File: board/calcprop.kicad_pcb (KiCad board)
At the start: 2 copper layers, 86.6 x 171.6 mm, 126 parts, among them CON1 SD_Card, P1 BATT, P10 PROG, P2 POWER, P3 EXTBATT, P5 BACKLIGHT, P6 DISPLAY, P7 FPU, P8 EXTSPI, P9 EXTIO, SW1 KEY, SW10 KEY, SW11 KEY, SW12 KEY, SW13 KEY, SW14 KEY, SW15 KEY, SW16 KEY, SW17 KEY, SW18 KEY, SW19 KEY, SW2 KEY, SW20 KEY, SW21 KEY, SW22 KEY, SW23 KEY, SW24 KEY, SW25 KEY, SW26 KEY, SW27 KEY, SW28 KEY, SW29 KEY, SW3 KEY, SW30 KEY, SW31 KEY, SW32 KEY, SW33 KEY, SW34 KEY, SW35 KEY, SW36 KEY, SW37 KEY, SW38 KEY, SW39 KEY, SW4 KEY, SW40 KEY, SW41 KEY, SW42 KEY, SW43 KEY, SW44 KEY, SW45 KEY, SW46 KEY, SW47 KEY, SW48 KEY, SW5 KEY, SW6 KEY, SW7 KEY, SW8 KEY, SW9 KEY, U1 74LS595, U2 PROPELLER-QFN, U3 MCP3002, U4 LTC3525-3.3, U5 24LC512, U6 SST25VF080, U7 MCP23S17, U8 23xx1024, U9 23xx1024, Y1 5MHz

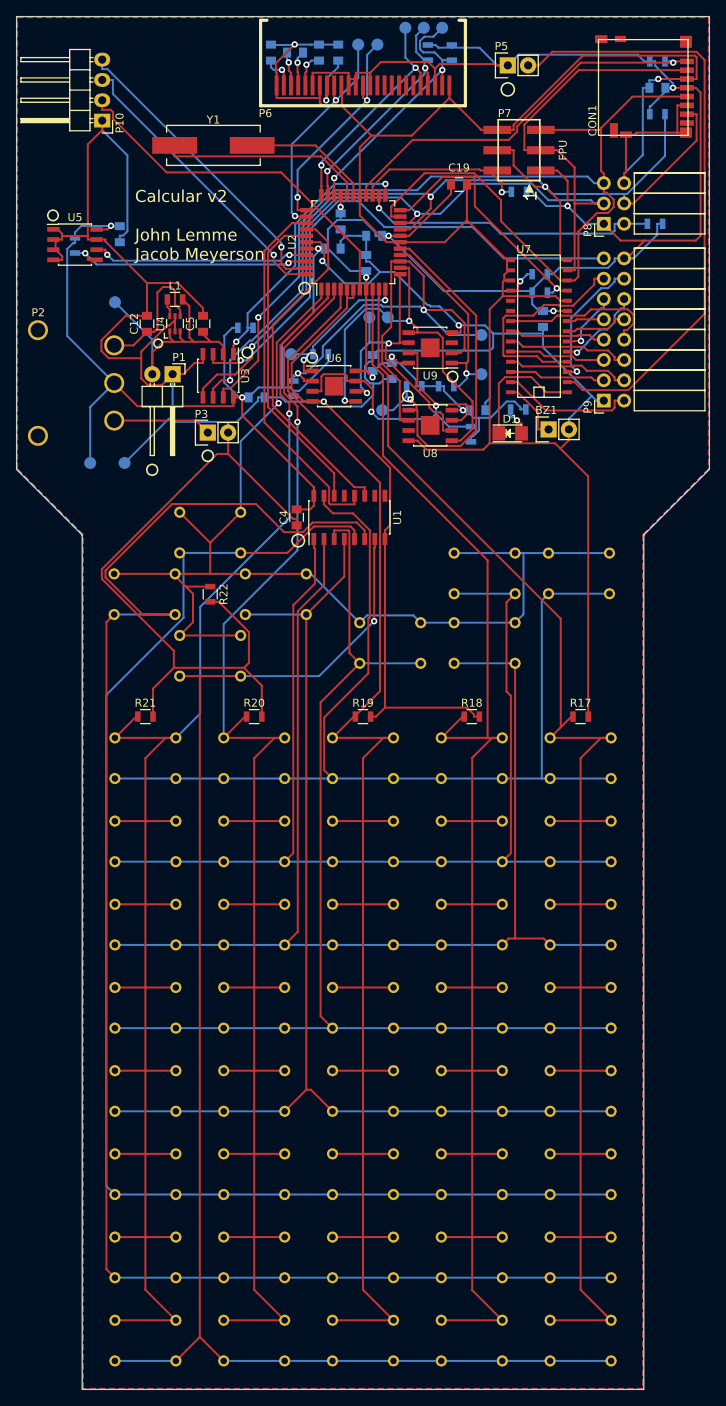
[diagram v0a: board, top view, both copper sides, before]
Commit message: First draft of case
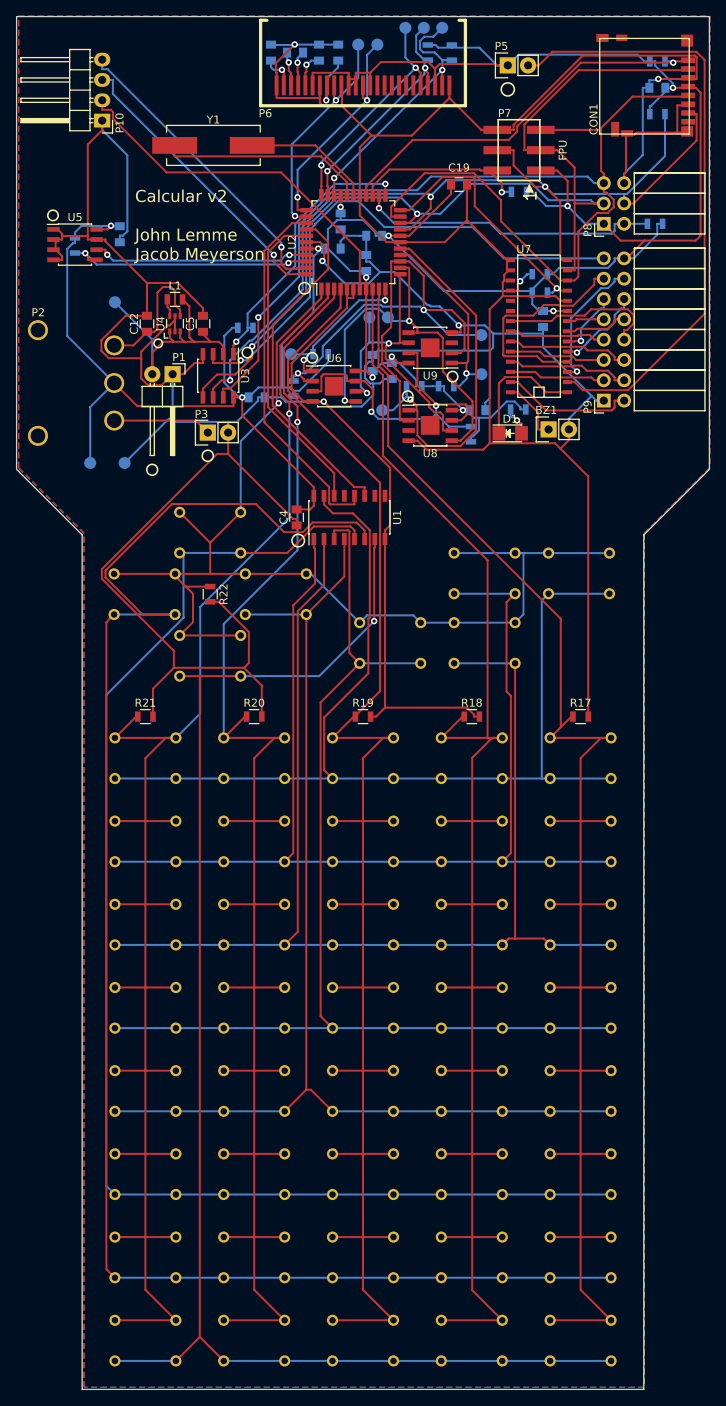
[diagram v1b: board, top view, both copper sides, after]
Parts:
- moved CON1 0.21 mm to (109.2, 31.4)
